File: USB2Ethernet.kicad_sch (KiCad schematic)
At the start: 33 parts, among them J8 USB_A_Stacked, U16 LAN9514, U17 CAT250xxx, Y5 25Mhz

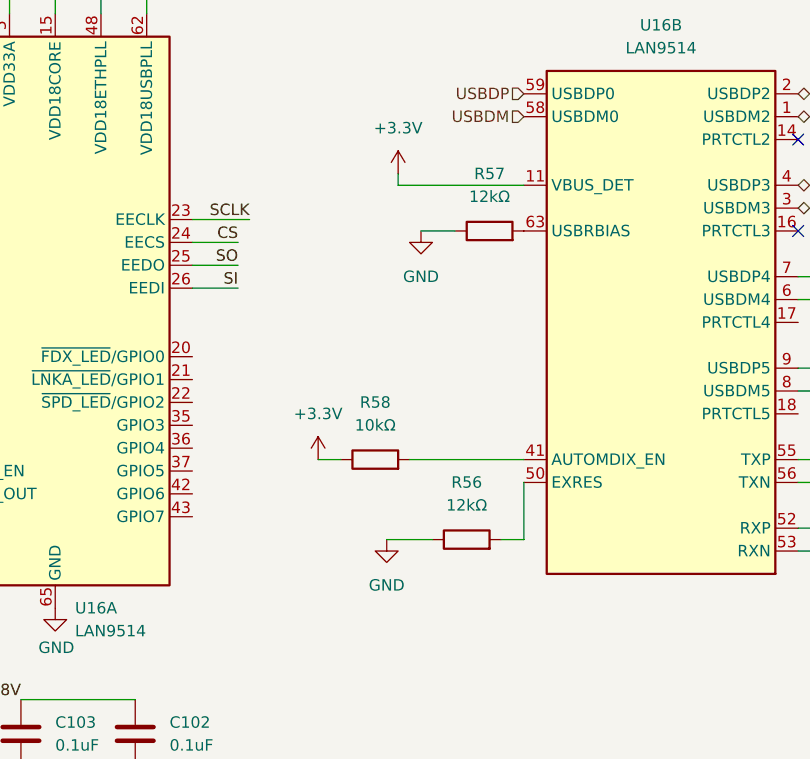
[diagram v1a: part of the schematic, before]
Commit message: change design
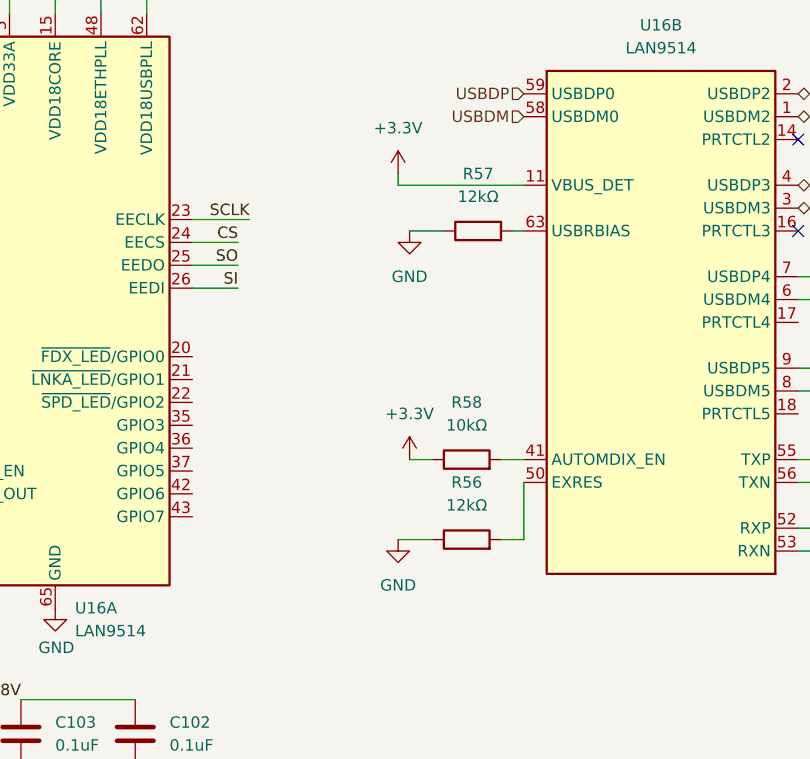
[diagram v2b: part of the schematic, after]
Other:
- moved on the sheet: R57, R58
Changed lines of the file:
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@@
 	(wire
 		(pts
-			(xy 132.08 100.33) (xy 144.78 100.33)
+			(xy 142.24 100.33) (xy 144.78 100.33)
 		)
 		(stroke
@@
 	(wire
 		(pts
-			(xy 133.35 74.93) (xy 137.16 74.93)
+			(xy 132.08 74.93) (xy 135.89 74.93)
 		)
 		(stroke
@@
 	(wire
 		(pts
-			(xy 121.92 100.33) (xy 124.46 100.33)
+			(xy 132.08 100.33) (xy 134.62 100.33)
 		)
 		(stroke
@@
 	(wire
 		(pts
+			(xy 143.51 74.93) (xy 144.78 74.93)
+		)
+		(stroke
+			(width 0)
+			(type default)
+		)
+	)
+	(wire
+		(pts
 			(xy 58.42 119.38) (xy 58.42 114.3)
 		)
@@
 	(wire
 		(pts
-			(xy 129.54 109.22) (xy 134.62 109.22)
+			(xy 130.81 109.22) (xy 134.62 109.22)
 		)
 		(stroke
@@
 	(label "SI"
 		(at 113.03 81.28 180)
+		(fields_autoplaced yes)
 		(effects
 			(font
@@
 	(label "1.8V"
 		(at 92.71 45.72 180)
+		(fields_autoplaced yes)
 		(effects
 			(font
@@
 	(label "USB5DN"
 		(at 259.08 97.79 180)
+		(fields_autoplaced yes)
 		(effects
 			(font
@@
 	(label "USB4DN"
 		(at 259.08 102.87 180)
+		(fields_autoplaced yes)
 		(effects
 			(font
@@
 	(label "USB4DP"
 		(at 184.15 80.01 180)
+		(fields_autoplaced yes)
 		(effects
 			(font
@@
 	(label "USB5DP"
 		(at 184.15 90.17 180)
+		(fields_autoplaced yes)
 		(effects
 			(font
@@
 	(label "SO"
 		(at 68.58 26.67 180)
+		(fields_autoplaced yes)
 		(effects
 			(font
@@
 	(label "VDDA"
 		(at 87.63 48.26 180)
+		(fields_autoplaced yes)
 		(effects
 			(font
@@
 	(label "CS"
 		(at 36.83 26.67 0)
+		(fields_autoplaced yes)
 		(effects
 			(font
@@
 	(label "SCLK"
 		(at 69.85 21.59 180)
+		(fields_autoplaced yes)
 		(effects
 			(font
@@
 	(label "USB5DN"
 		(at 184.15 92.71 180)
+		(fields_autoplaced yes)
 		(effects
 			(font
@@
 	(label "CS"
 		(at 113.03 76.2 180)
+		(fields_autoplaced yes)
 		(effects
 			(font
@@
 	(label "USB4DN"
 		(at 184.15 82.55 180)
+		(fields_autoplaced yes)
 		(effects
 			(font
@@
 	(label "VDDA"
 		(at 101.6 146.05 0)
+		(fields_autoplaced yes)
 		(effects
 			(font
@@
 	(label "USB4DP"
 		(at 259.08 100.33 180)
+		(fields_autoplaced yes)
 		(effects
 			(font
@@
 	(label "VDDIO"
 		(at 82.55 50.8 180)
+		(fields_autoplaced yes)
 		(effects
 			(font
@@
 	(label "SCLK"
 		(at 114.3 73.66 180)
+		(fields_autoplaced yes)
 		(effects
 			(font
@@
 	(label "1.8V"
 		(at 88.9 127 180)
+		(fields_autoplaced yes)
 		(effects
 			(font
@@
 	(label "SI"
 		(at 68.58 24.13 180)
+		(fields_autoplaced yes)
 		(effects
 			(font
@@
 	(label "SO"
 		(at 113.03 78.74 180)
+		(fields_autoplaced yes)
 		(effects
 			(font
@@
 	(label "VDDA"
 		(at 193.04 83.82 180)
+		(fields_autoplaced yes)
 		(effects
 			(font
@@
 	(label "VDDIO"
 		(at 90.17 168.91 0)
+		(fields_autoplaced yes)
 		(effects
 			(font
@@
 	(label "USB5DP"
 		(at 259.08 95.25 180)
+		(fields_autoplaced yes)
 		(effects
 			(font
@@
 		(shape bidirectional)
 		(at 175.26 59.69 0)
+		(fields_autoplaced yes)
 		(effects
 			(font
@@
 		(shape bidirectional)
 		(at 175.26 69.85 0)
+		(fields_autoplaced yes)
 		(effects
 			(font
@@
 		(shape input)
 		(at 259.08 87.63 180)
+		(fields_autoplaced yes)
 		(effects
 			(font
@@
 		(shape output)
 		(at 226.06 102.87 0)
+		(fields_autoplaced yes)
 		(effects
 			(font
@@
 		(shape input)
 		(at 226.06 110.49 0)
+		(fields_autoplaced yes)
 		(effects
 			(font
@@
 		(shape bidirectional)
 		(at 175.26 72.39 0)
+		(fields_autoplaced yes)
 		(effects
 			(font
@@
 		(shape bidirectional)
 		(at 175.26 62.23 0)
+		(fields_autoplaced yes)
 		(effects
 			(font
@@
 		(shape input)
 		(at 226.06 107.95 0)
+		(fields_autoplaced yes)
 		(effects
 			(font
@@
 		(shape input)
 		(at 73.66 68.58 180)
+		(fields_autoplaced yes)
 		(effects
 			(font
@@
 		(shape output)
 		(at 226.06 100.33 0)
+		(fields_autoplaced yes)
 		(effects
 			(font
@@
 		(shape input)
 		(at 144.78 59.69 180)
+		(fields_autoplaced yes)
 		(effects
 			(font
@@
 		(shape input)
 		(at 144.78 62.23 180)
+		(fields_autoplaced yes)
 		(effects
 			(font
@@
 	(symbol
 		(lib_id "Device:R")
-		(at 128.27 100.33 90)
+		(at 138.43 100.33 90)
 		(unit 1)
 		(exclude_from_sim no)
@@
 		(fields_autoplaced yes)
 		(property "Reference" "R58"
-			(at 128.27 93.98 90)
+			(at 138.43 93.98 90)
 			(effects
 				(font
@@
 		)
 		(property "Value" "10kΩ"
-			(at 128.27 96.52 90)
+			(at 138.43 96.52 90)
 			(effects
 				(font
@@
 		)
 		(property "Footprint" "Resistor_SMD:R_0603_1608Metric_Pad0.98x0.95mm_HandSolder"
-			(at 128.27 102.108 90)
+			(at 138.43 102.108 90)
 			(effects
 				(font
@@
 		)
 		(property "Datasheet" "~"
-			(at 128.27 100.33 0)
+			(at 138.43 100.33 0)
 			(effects
 				(font
@@
 		)
 		(property "Description" "Resistor"
-			(at 128.27 100.33 0)
+			(at 138.43 100.33 0)
 			(effects
 				(font
@@
 	(symbol
 		(lib_id "power:GND")
-		(at 133.35 74.93 0)
+		(at 132.08 74.93 0)
 		(unit 1)
 		(exclude_from_sim no)
@@
 		(fields_autoplaced yes)
 		(property "Reference" "#PWR0808"
-			(at 133.35 81.28 0)
+			(at 132.08 81.28 0)
 			(effects
 				(font
@@
 		)
 		(property "Value" "GND"
-			(at 133.35 80.01 0)
+			(at 132.08 80.01 0)
 			(effects
 				(font
@@
 		)
 		(property "Footprint" ""
-			(at 133.35 74.93 0)
+			(at 132.08 74.93 0)
 			(effects
 				(font
@@
 		)
 		(property "Datasheet" ""
-			(at 133.35 74.93 0)
+			(at 132.08 74.93 0)
 			(effects
 				(font
@@
 		)
 		(property "Description" "Power symbol creates a global label with name \"GND\" , ground"
-			(at 133.35 74.93 0)
+			(at 132.08 74.93 0)
 			(effects
 				(font
@@
 	(symbol
 		(lib_id "power:GND")
-		(at 129.54 109.22 0)
+		(at 130.81 109.22 0)
 		(unit 1)
 		(exclude_from_sim no)
@@
 		(fields_autoplaced yes)
 		(property "Reference" "#PWR0809"
-			(at 129.54 115.57 0)
+			(at 130.81 115.57 0)
 			(effects
 				(font
@@
 		)
 		(property "Value" "GND"
-			(at 129.54 114.3 0)
+			(at 130.81 114.3 0)
 			(effects
 				(font
@@
 		)
 		(property "Footprint" ""
-			(at 129.54 109.22 0)
+			(at 130.81 109.22 0)
 			(effects
 				(font
@@
 		)
 		(property "Datasheet" ""
-			(at 129.54 109.22 0)
+			(at 130.81 109.22 0)
 			(effects
 				(font
@@
 		)
 		(property "Description" "Power symbol creates a global label with name \"GND\" , ground"
-			(at 129.54 109.22 0)
+			(at 130.81 109.22 0)
 			(effects
 				(font
@@
 	(symbol
 		(lib_id "power:+3.3V")
-		(at 121.92 100.33 0)
+		(at 132.08 100.33 0)
 		(unit 1)
 		(exclude_from_sim no)
@@
 		(fields_autoplaced yes)
 		(property "Reference" "#PWR040"
-			(at 121.92 104.14 0)
+			(at 132.08 104.14 0)
 			(effects
 				(font
@@
 		)
 		(property "Value" "+3.3V"
-			(at 121.92 95.25 0)
+			(at 132.08 95.25 0)
 			(effects
 				(font
@@
 		)
 		(property "Footprint" ""
-			(at 121.92 100.33 0)
+			(at 132.08 100.33 0)
 			(effects
 				(font
@@
 		)
 		(property "Datasheet" ""
-			(at 121.92 100.33 0)
+			(at 132.08 100.33 0)
 			(effects
 				(font
@@
 		)
 		(property "Description" "Power symbol creates a global label with name \"+3.3V\""
-			(at 121.92 100.33 0)
+			(at 132.08 100.33 0)
 			(effects
 				(font
@@
 	(symbol
 		(lib_id "Device:R")
-		(at 140.97 74.93 90)
+		(at 139.7 74.93 90)
 		(unit 1)
 		(exclude_from_sim no)
@@
 		(fields_autoplaced yes)
 		(property "Reference" "R57"
-			(at 140.97 68.58 90)
+			(at 139.7 68.58 90)
 			(effects
 				(font
@@
 		)
 		(property "Value" "12kΩ"
-			(at 140.97 71.12 90)
+			(at 139.7 71.12 90)
 			(effects
 				(font
@@
 		)
 		(property "Footprint" "Resistor_SMD:R_0603_1608Metric_Pad0.98x0.95mm_HandSolder"
-			(at 140.97 76.708 90)
+			(at 139.7 76.708 90)
 			(effects
 				(font
@@
 		)
 		(property "Datasheet" "~"
-			(at 140.97 74.93 0)
+			(at 139.7 74.93 0)
 			(effects
 				(font
@@
 		)
 		(property "Description" "Resistor"
-			(at 140.97 74.93 0)
+			(at 139.7 74.93 0)
 			(effects
 				(font
